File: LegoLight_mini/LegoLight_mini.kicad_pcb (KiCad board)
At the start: 2 copper layers, 11.2 x 26.2 mm, 6 parts, among them J1 Conn_02x04_Odd_Even, J2 +bat, SW1 SW_Push, U1 ATtiny402-SS

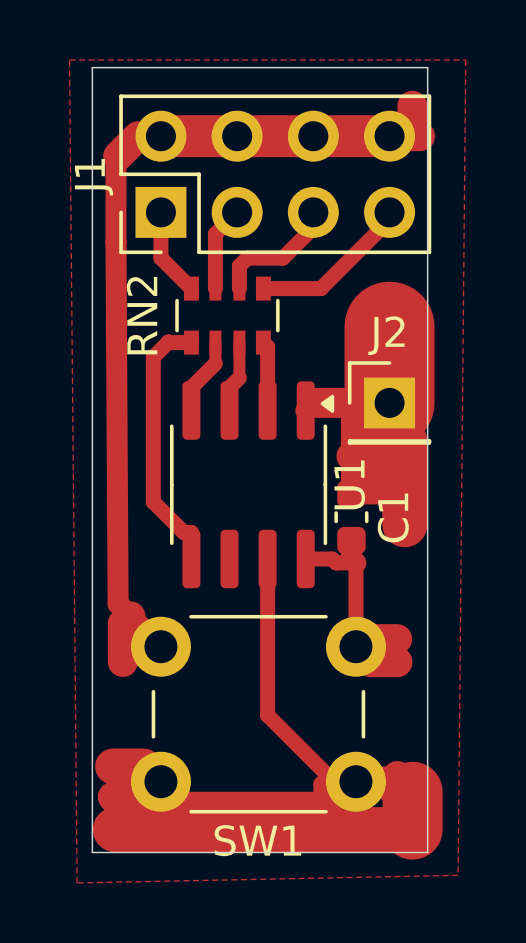
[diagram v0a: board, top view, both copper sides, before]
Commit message: adding freecad models
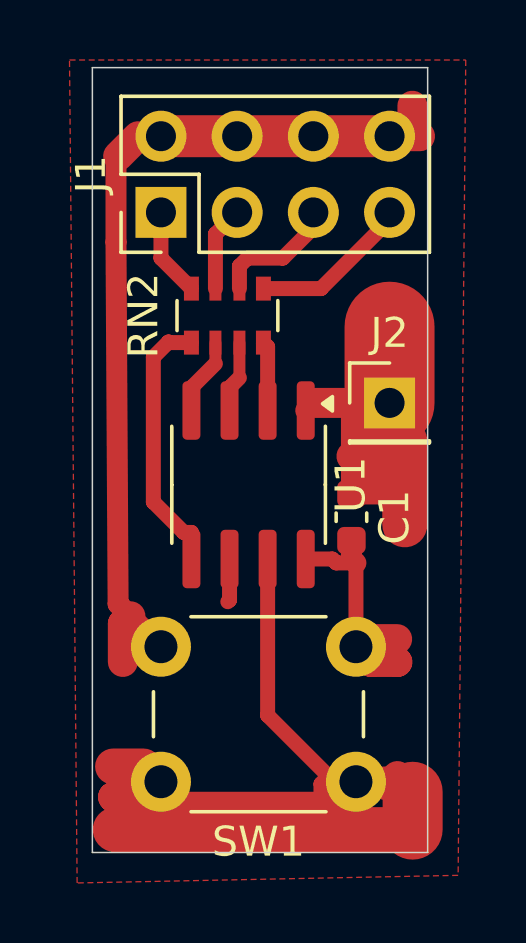
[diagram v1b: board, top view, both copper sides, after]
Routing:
- net /UPDI: track 0.00 -> 1.45 mm
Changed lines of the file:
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@@
 			(psa4output no)
 			(plot_black_and_white yes)
-			(plotinvisibletext no)
 			(sketchpadsonfab no)
 			(plotpadnumbers no)
@@
 		(net 11)
 	)
+	(segment
+		(start 111.539 104.4372)
+		(end 111.4806 104.4956)
+		(width 0.5)
+		(layer "F.Cu")
+		(net 12)
+	)
+	(segment
+		(start 111.539 103.072)
+		(end 111.539 104.4372)
+		(width 0.5)
+		(layer "F.Cu")
+		(net 12)
+	)
 	(zone
 		(net 7)
@@
 		(hatch edge 0.5)
 		(connect_pads
-			(clearance 0.8)
+			(clearance 0.7)
 		)
 		(min_thickness 0.25)
